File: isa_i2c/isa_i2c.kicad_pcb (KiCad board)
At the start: 4 copper layers, 99.9 x 87.1 mm, 27 parts, among them J10 Conn_01x04, J12 Conn_01x04, J13 Conn_01x04, J14 Conn_01x04, J15 Conn_01x04, J16 Conn_01x04, J8 Bus_ISA_8bit, Q1 BS170, Q2 BS250, SW1 SW_DIP_x08, U2 74HC245, U3 PCF8584, U7 74HCT688

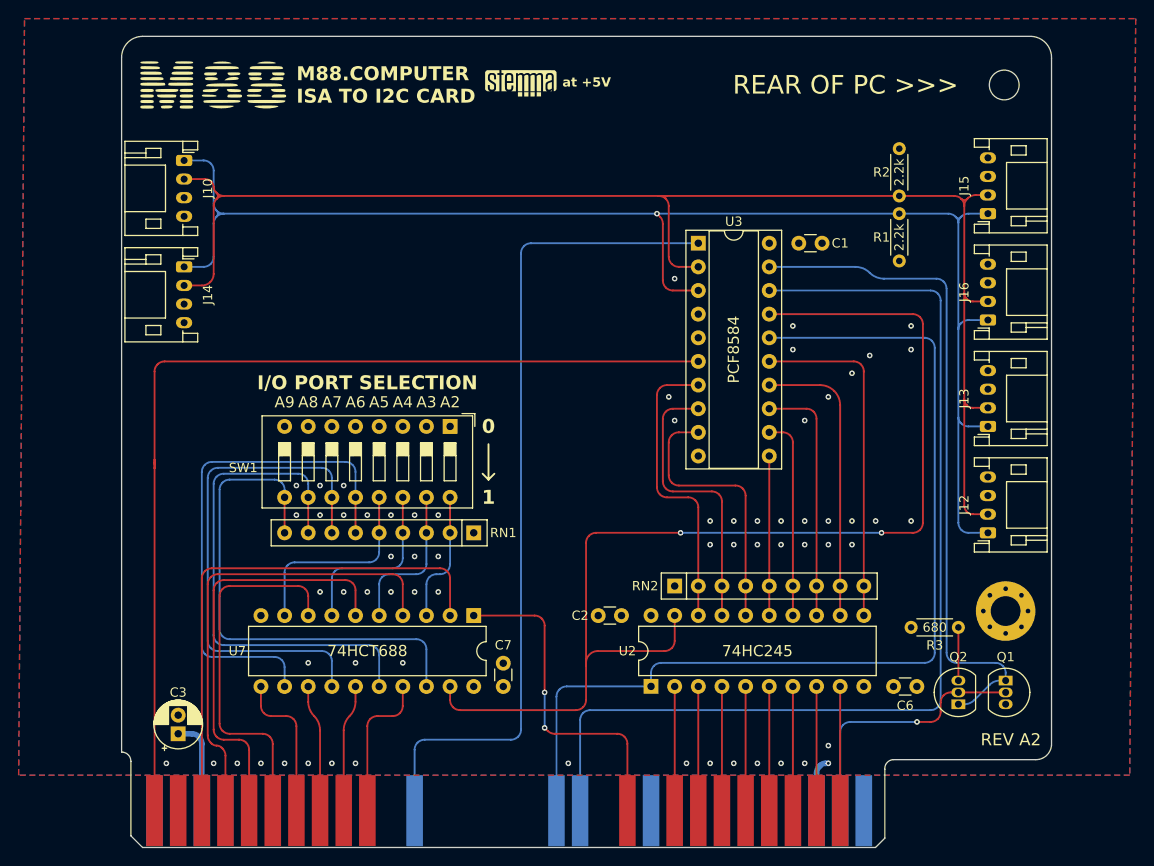
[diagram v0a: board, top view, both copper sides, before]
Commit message: motherboard tweaks for manufacturing run, i2c card tweaks for manufacturing run, de9 -> stemma adapter idea for the i2c card
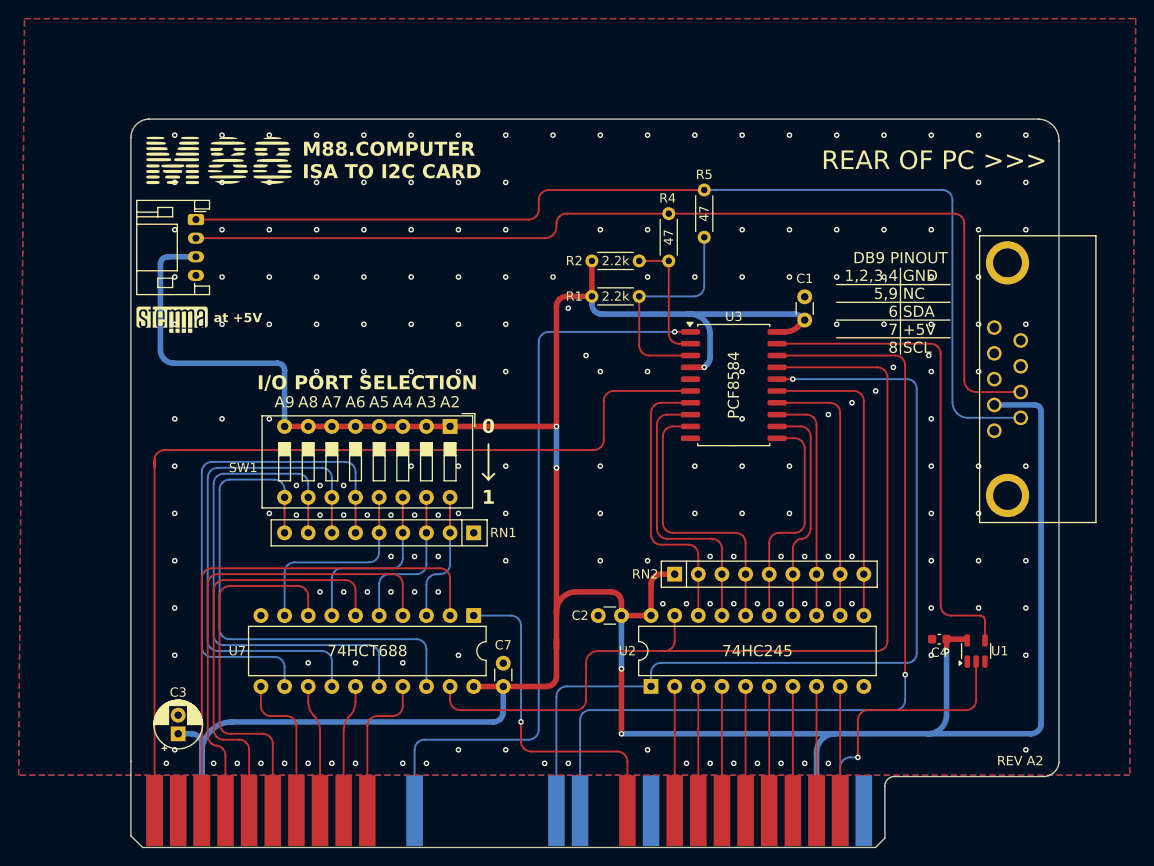
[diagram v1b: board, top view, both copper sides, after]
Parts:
- removed C6: 0.1 uF, Capacitor_THT:C_Disc_D3.0mm_W1.6mm_P2.50mm
- removed H1: MountingHole, MountingHole:MountingHole_3.2mm_M3
- removed H2: MountingHole_Pad, MountingHole:MountingHole_3.2mm_M3_Pad_Via
- removed J12, J13, J14, J15, J16: Conn_01x04, Connector_JST:JST_PH_S4B-PH-K_1x04_P2.00mm_Horizontal
- removed Q1: BS170, Package_TO_SOT_THT:TO-92_Inline
- removed Q2: BS250, Package_TO_SOT_THT:TO-92_Inline
- removed R3: 680 1/8W, Resistor_THT:R_Axial_DIN0204_L3.6mm_D1.6mm_P5.08mm_Horizontal
- added C4: 0.1 uF, Capacitor_SMD:C_0603_1608Metric, F.Cu at (182.1, 111.1)
- added J1: DE9_Receptacle, SamacSys_Parts:L77SDE09SA4CH4F, F.Cu at (188.0, 77.6)
- added R4: 47 1/8W, Resistor_THT:R_Axial_DIN0204_L3.6mm_D1.6mm_P5.08mm_Horizontal, F.Cu at (153.0, 70.5)
- added R5: 47 1/8W, Resistor_THT:R_Axial_DIN0204_L3.6mm_D1.6mm_P5.08mm_Horizontal, F.Cu at (156.8, 67.9)
- added U1: 74AHC1G04, Package_TO_SOT_SMD:SOT-23-5, F.Cu at (186.1, 112.4)
- U3: footprint Package_DIP:DIP-20_W7.62mm_Socket -> Package_SO:SOIC-20W_7.5x12.8mm_P1.27mm
- moved G*** 45.3 mm to (99.7, 76.8)
- moved R1 29.3 mm to (149.9, 74.3), turned to 180 degrees
- moved R2 28.8 mm to (149.9, 70.5), turned to 180 degrees
- moved U3 15.7 mm to (160.0, 83.8)
- moved C1 8.28 mm to (167.6, 76.8), turned to 90 degrees
- moved G*** 8.13 mm to (104.8, 59.7)
- moved J10 6.48 mm to (102.2, 66.0)
- moved RN2 1.27 mm to (153.7, 104.1)
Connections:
- R1 pad 1: /SCL -> /PCF_SCL
- R2 pad 1: /SDA -> /PCF_SDA
- U3 pad 2: /SDA -> /PCF_SDA
- U3 pad 3: /SCL -> /PCF_SCL
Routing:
- net +5V: track 16.2 -> 352.1 mm, vias 1 -> 6
- net /SDA: track 156.1 -> 108.4 mm
- net /SCL: track 157.5 -> 114.1 mm, vias 1 -> 0
- net /PCF_SCL: track 0.00 -> 24.2 mm
- net /~{CS}: track 124.0 -> 100.3 mm, vias 2 -> 0
- net /~{RESET}: track 72.2 -> 53.0 mm
- net /~{IOW}: track 111.6 -> 96.2 mm, vias 0 -> 1
- net /PCF_SDA: track 0.00 -> 13.6 mm
- net /CLK: track 90.0 -> 79.6 mm, vias 0 -> 1
- net /~{IOR}: track 107.3 -> 98.2 mm, vias 0 -> 1
- net /D3: track 17.1 -> 24.4 mm
- net Net-(Q2-S): track 5.71 -> 0.00 mm
- net /BA00: track 107.1 -> 102.0 mm
- net /D7: track 37.0 -> 33.0 mm
- net /D4: track 21.7 -> 24.4 mm
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- removed copper zone on In1.Cu, net +5V
- removed copper zone on In2.Cu, net GND
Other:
- board size 99.9 x 87.1 mm -> 99.7 x 78.3 mm
- copper layers 4 -> 2
- board text added: "1,2,3,4 5,9 6 7 8"
- board text added: "47"
- board text added: "DB9 PINOUT"
- board text added: "GND NC SDA +5V SCL"
- board text added: "TOP OF BRACKET"
- board text removed: "680"
